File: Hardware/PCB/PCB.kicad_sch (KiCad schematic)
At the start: 72 parts, among them CN1 XT30UPB-M, J1 Connector, USB-TYPE-C-16P, SW1 TS-1187A-B-A-B, U1 RP2350B_C42415655, U10 KF128-2.54-3P, U11 KF128-2.54-3P, U12 KF128-2.54-3P, U2 KF128-2.54-2P, U3 BMP581, U4 ICM-45686, U5 BQ25883RGER, U6 LMR51430YFDDCR, U7 TPS630701RNMR, U8 GD25Q128ESIGR, U9 KF128-2.54-3P, X2 X322512MSB4SI

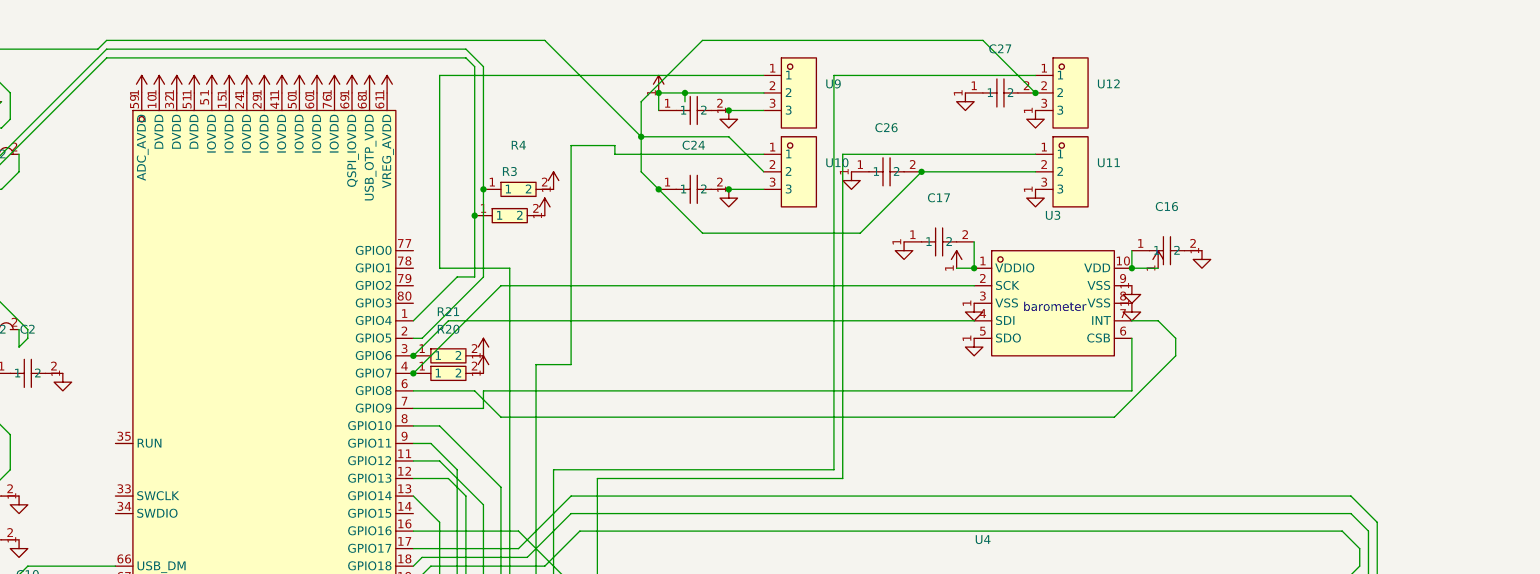
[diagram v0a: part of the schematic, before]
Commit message: Restarting PCB, finished Flash memory application
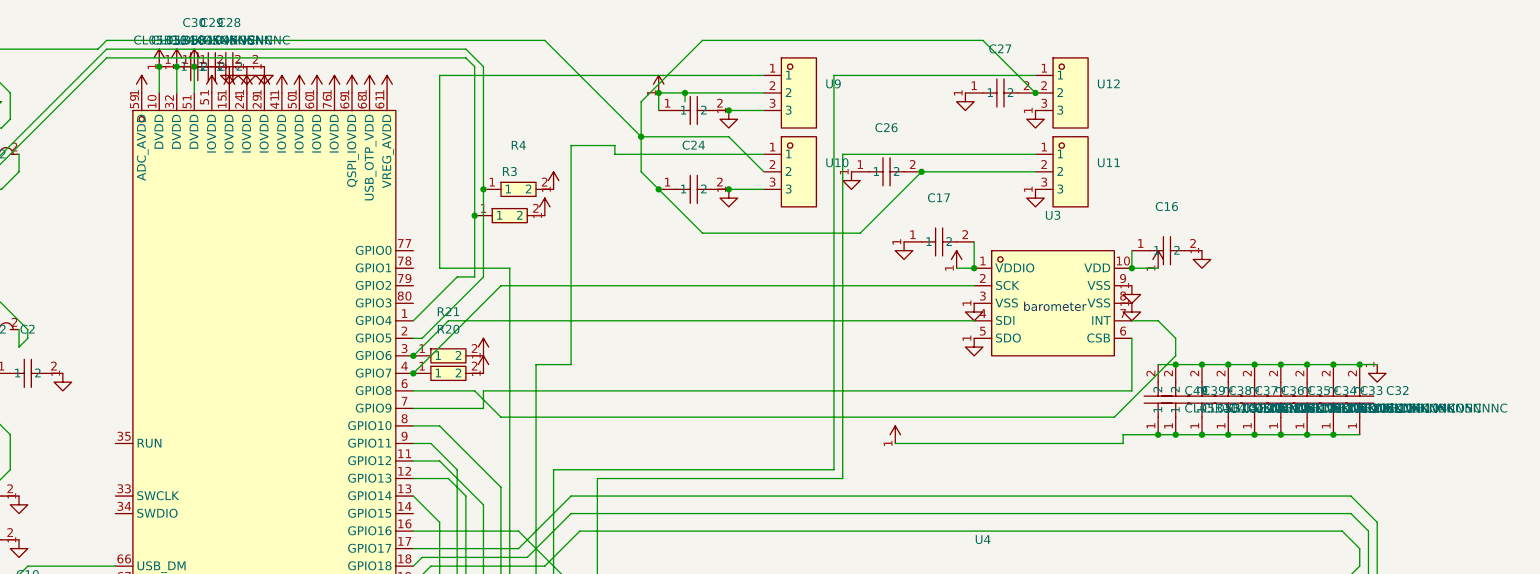
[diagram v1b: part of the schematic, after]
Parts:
- added C28, C29, C30, C32, C33, C34, C35, C36, C37, C38, C39, C40: CL05B104KO5NNNC, easyeda2kicad:C0402, symbol easyeda2kicad:CL05B104KO5NNNC
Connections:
- net +1V1: now also C28.1, C29.1, C30.1
- net +3V3: now also C32.1, C33.1, C34.1, C35.1, C36.1, C37.1, C38.1, C39.1, C40.1
- net GND: now also C28.2, C29.2, C30.2, C32.2, C33.2, C34.2, C35.2, C36.2, C37.2, C38.2, C39.2, C40.2
